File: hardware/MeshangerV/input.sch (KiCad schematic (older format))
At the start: 26 parts

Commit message: more schematic
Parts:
- U?: symbol Useful_ICs:SN3218 -> MeshangerV-rescue:SN3218-Useful_ICs
- U?: symbol Useful_ICs:AT42QT2120 -> MeshangerV-rescue:AT42QT2120-Useful_ICs
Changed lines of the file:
@@
 EESchema Schematic File Version 4
 LIBS:MeshangerV-cache
-EELAYER 29 0
+EELAYER 26 0
 EELAYER END
 $Descr A4 11693 8268
 encoding utf-8
-Sheet 3 3
+Sheet 3 4
 Title ""
 Date ""
@@
 GND
 $Comp
-L Useful_ICs:SN3218 U?
+L MeshangerV-rescue:SN3218-Useful_ICs U?
 U 1 1 5FE09172
 P 2850 4250
@@
 $EndComp
 $Comp
-L Useful_ICs:AT42QT2120 U?
+L MeshangerV-rescue:AT42QT2120-Useful_ICs U?
 U 1 1 5FE0B088
 P 6750 1700

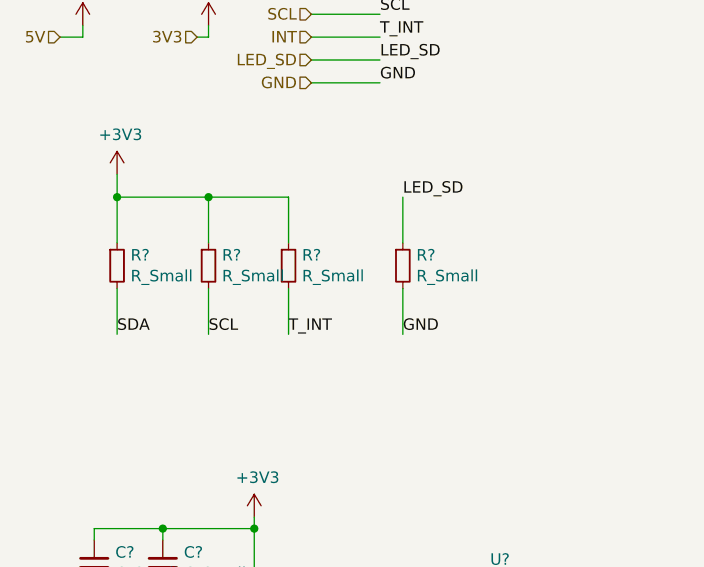
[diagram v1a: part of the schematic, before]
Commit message: schematic complete more or less
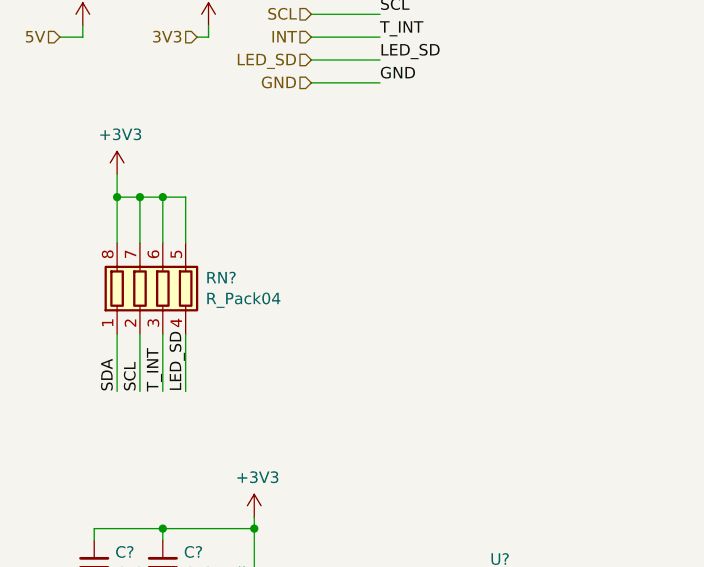
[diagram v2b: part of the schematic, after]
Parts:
- removed R? (x4): R_Small, symbol Device:R_Small
- added RN?: R_Pack04, symbol Device:R_Pack04
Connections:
- net +3V3: now also RN?.5 (R4.2), RN?.6 (R3.2), RN?.7 (R2.2), RN?.8 (R1.2)
- net INT: now also RN?.3 (R3.1)
- net LED_SD: now also RN?.4 (R4.1)
- net SCL: now also RN?.2 (R2.1)
- net SDA: now also RN?.1 (R1.1)
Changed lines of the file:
@@
 EESchema Schematic File Version 4
 LIBS:MeshangerV-cache
-EELAYER 26 0
+EELAYER 29 0
 EELAYER END
 $Descr A4 11693 8268
 encoding utf-8
-Sheet 3 4
+Sheet 3 5
 Title ""
 Date ""
@@
 GND
 $Comp
-L Device:R_Small R?
-U 1 1 5FEC910A
-P 1550 1850
-F 0 "R?" H 1609 1896 50  0000 L CNN
-F 1 "R_Small" H 1609 1805 50  0000 L CNN
-F 2 "" H 1550 1850 50  0001 C CNN
-F 3 "~" H 1550 1850 50  0001 C CNN
-	1    1550 1850
-	1    0    0    -1
-$EndComp
-$Comp
-L Device:R_Small R?
-U 1 1 5FEC96E3
-P 1150 1850
-F 0 "R?" H 1209 1896 50  0000 L CNN
-F 1 "R_Small" H 1209 1805 50  0000 L CNN
-F 2 "" H 1150 1850 50  0001 C CNN
-F 3 "~" H 1150 1850 50  0001 C CNN
-	1    1150 1850
-	1    0    0    -1
-$EndComp
-$Comp
 L power:+3V3 #PWR?
 U 1 1 5FEC9D64
@@
 Wire Wire Line
 	5700 800  5700 650
-$Comp
-L Device:R_Small R?
-U 1 1 5FED518F
-P 1900 1850
-F 0 "R?" H 1959 1896 50  0000 L CNN
-F 1 "R_Small" H 1959 1805 50  0000 L CNN
-F 2 "" H 1900 1850 50  0001 C CNN
-F 3 "~" H 1900 1850 50  0001 C CNN
-	1    1900 1850
-	1    0    0    -1
-$EndComp
 Wire Wire Line
 	1150 1750 1150 1550
 Wire Wire Line
-	1150 1550 1550 1550
-Wire Wire Line
-	1550 1550 1550 1750
+	1150 1550 1250 1550
+Wire Wire Line
+	1250 1550 1250 1750
 Connection ~ 1150 1550
 Wire Wire Line
 	1150 1550 1150 1450
 Wire Wire Line
-	1550 1550 1900 1550
-Wire Wire Line
-	1900 1550 1900 1750
-Connection ~ 1550 1550
-Wire Wire Line
-	1150 1950 1150 2150
-Wire Wire Line
-	1550 1950 1550 2150
-Wire Wire Line
-	1900 1950 1900 2150
-Text Label 1550 2150 0    50   ~ 0
+	1250 1550 1350 1550
+Wire Wire Line
+	1350 1550 1350 1750
+Connection ~ 1250 1550
+Text Label 1250 2400 1    50   ~ 0
 SCL
-Text Label 1900 2150 0    50   ~ 0
+Text Label 1350 2400 1    50   ~ 0
 T_INT
-Text Label 1150 2150 0    50   ~ 0
+Text Label 1150 2400 1    50   ~ 0
 SDA
 $Comp
@@
 Wire Wire Line
 	2000 1050 2300 1050
-$Comp
-L Device:R_Small R?
-U 1 1 5FF2D759
-P 2400 1850
-F 0 "R?" H 2459 1896 50  0000 L CNN
-F 1 "R_Small" H 2459 1805 50  0000 L CNN
-F 2 "" H 2400 1850 50  0001 C CNN
-F 3 "~" H 2400 1850 50  0001 C CNN
-	1    2400 1850
-	1    0    0    -1
-$EndComp
-Wire Wire Line
-	2400 1750 2400 1550
-Wire Wire Line
-	2400 1950 2400 2150
-Text Label 2400 2150 0    50   ~ 0
-GND
-Text Label 2400 1550 0    50   ~ 0
+Wire Wire Line
+	1450 1750 1450 1550
+Text Label 1450 2400 1    50   ~ 0
 LED_SD
+Wire Wire Line
+	1350 1550 1450 1550
+Connection ~ 1350 1550
+$Comp
+L Device:R_Pack04 RN?
+U 1 1 5FEA8355
+P 1350 1950
+AR Path="/5FEA8355" Ref="RN?"  Part="1"
+AR Path="/5FDFCE72/5FEA8355" Ref="RN?"  Part="1"
+F 0 "RN?" H 1538 1996 50  0000 L CNN
+F 1 "R_Pack04" H 1538 1905 50  0000 L CNN
+F 2 "" V 1625 1950 50  0001 C CNN
+F 3 "~" H 1350 1950 50  0001 C CNN
+	1    1350 1950
+	1    0    0    -1
+$EndComp
+Wire Wire Line
+	1150 2400 1150 2150
+Wire Wire Line
+	1250 2400 1250 2150
+Wire Wire Line
+	1350 2400 1350 2150
+Wire Wire Line
+	1450 2400 1450 2150
 $EndSCHEMATC
